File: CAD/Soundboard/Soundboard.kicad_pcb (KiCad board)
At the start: 2 copper layers, 105 x 85 mm, 53 parts, among them J1 USB4085-GF-A_REVB, Q1 IRLML6401, Q2 IRLML6401, Q3 IRLML6401, Q4 IRLML6401, SW1 SW_SPST, SW10 SW_SPST, SW11 SW_SPST, SW12 SW_SPST, SW13 SW_SPST, SW14 SW_SPST, SW15 SW_SPST, SW16 SW_SPST, SW2 SW_SPST, SW3 SW_SPST, SW4 SW_SPST, SW5 SW_SPST, SW6 SW_SPST, SW7 SW_SPST, SW8 SW_SPST, SW9 SW_SPST, U1 TLC59283DBQ

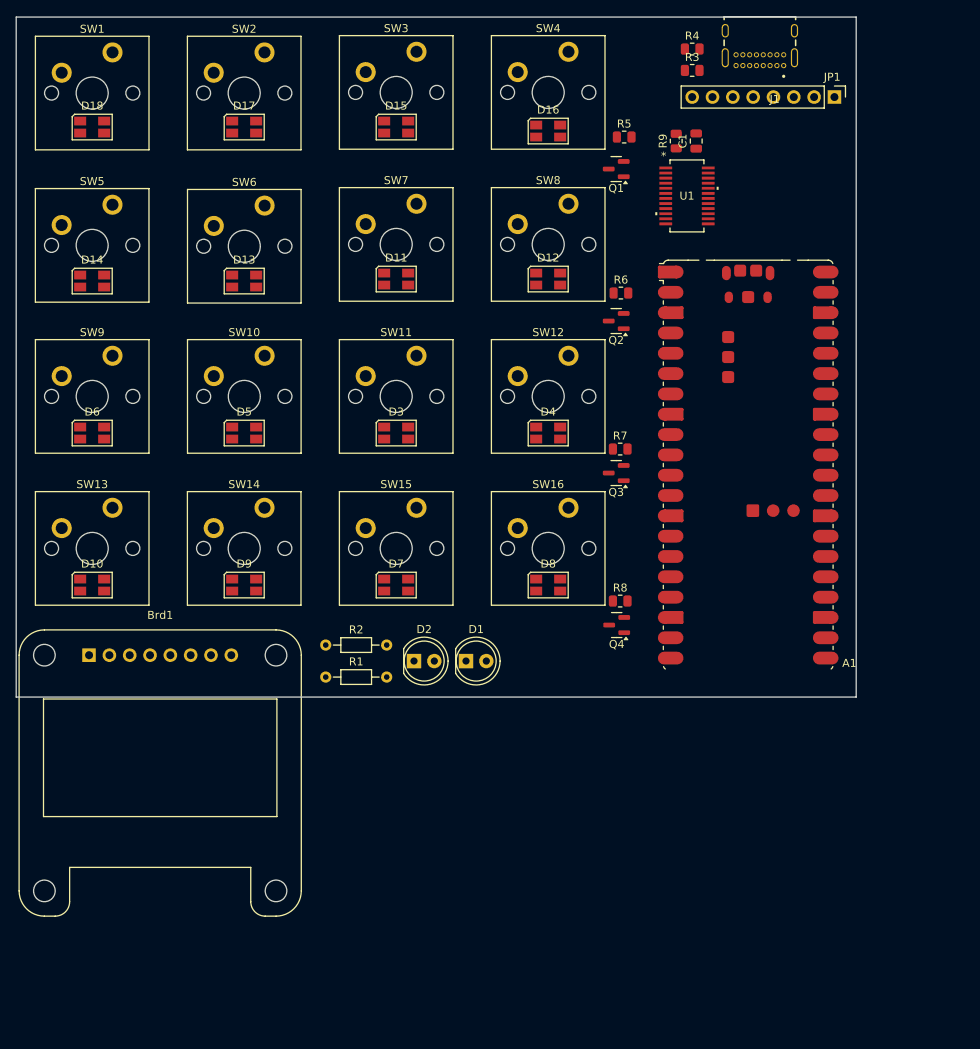
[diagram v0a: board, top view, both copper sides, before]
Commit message: do all the things
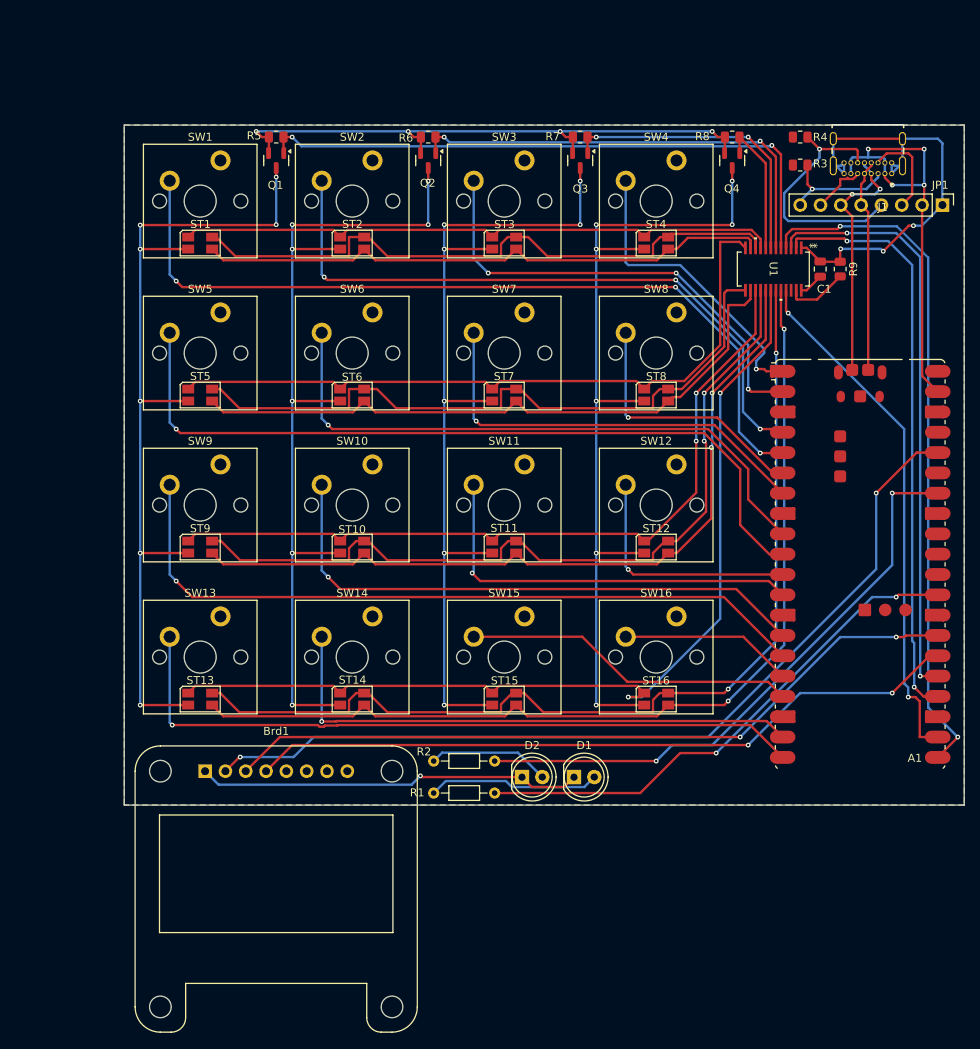
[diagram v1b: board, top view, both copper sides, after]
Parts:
- C1: value I dont know something big -> big
- J1: value USB4085-GF-A_REVB -> USB-C
- Q1, Q2: value IRLML6401 -> FET
- moved ST13 72.8 mm to (38.0, 100.2)
- moved ST16 71.9 mm to (95.0, 100.2)
- moved ST14 61.5 mm to (57.0, 100.2)
- moved ST15 61.3 mm to (76.0, 100.2)
- moved Q4 59.8 mm to (104.5, 32.9), turned to -90 degrees
- moved R8 59.7 mm to (104.5, 30.0)
- moved ST5 54.6 mm to (38.0, 62.2)
- moved ST4 53.7 mm to (95.0, 43.2)
- moved ST9 52.8 mm to (38.0, 81.2)
- moved ST12 51.7 mm to (95.0, 81.2)
- moved R5 43.5 mm to (47.5, 30.0)
- moved Q1 42.5 mm to (47.5, 32.9), turned to -90 degrees
- moved Q3 39.3 mm to (85.5, 32.9), turned to -90 degrees
- moved R7 39.3 mm to (85.5, 30.0)
- moved ST10 35.9 mm to (57.0, 81.2)
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- renumbered D15 to ST1, D13 to ST10, D5 to ST11, D9 to ST12, D18 to ST13, D14 to ST14, D6 to ST15, D10 to ST16, D11 to ST2, D3 to ST3, D7 to ST4, D16 to ST5, D12 to ST6, D4 to ST7, D8 to ST8, D17 to ST9
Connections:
- ST1 pad 1: Net-(D11-RK) -> Net-(ST1-RK)
- ST1 pad 2: Net-(D11-GK) -> Net-(ST1-GK)
- ST1 pad 3: Net-(D11-BK) -> Net-(ST1-BK)
- ST10 pad 1: Net-(D13-RK) -> Net-(ST10-RK)
- ST10 pad 2: Net-(D13-GK) -> Net-(ST10-GK)
- ST10 pad 3: Net-(D13-BK) -> Net-(ST10-BK)
- ST11 pad 1: Net-(D13-RK) -> Net-(ST10-RK)
- ST11 pad 2: Net-(D13-GK) -> Net-(ST10-GK)
- ST11 pad 3: Net-(D13-BK) -> Net-(ST10-BK)
- ST12 pad 1: Net-(D13-RK) -> Net-(ST10-RK)
- ST12 pad 2: Net-(D13-GK) -> Net-(ST10-GK)
- ST12 pad 3: Net-(D13-BK) -> Net-(ST10-BK)
- ST13 pad 1: Net-(D10-RK) -> Net-(ST13-RK)
- ST13 pad 2: Net-(D10-GK) -> Net-(ST13-GK)
- ST13 pad 3: Net-(D10-BK) -> Net-(ST13-BK)
- ST14 pad 1: Net-(D10-RK) -> Net-(ST13-RK)
- ST14 pad 2: Net-(D10-GK) -> Net-(ST13-GK)
- ST14 pad 3: Net-(D10-BK) -> Net-(ST13-BK)
- ST15 pad 1: Net-(D10-RK) -> Net-(ST13-RK)
- ST15 pad 2: Net-(D10-GK) -> Net-(ST13-GK)
- ST15 pad 3: Net-(D10-BK) -> Net-(ST13-BK)
- ST16 pad 1: Net-(D10-RK) -> Net-(ST13-RK)
- ST16 pad 2: Net-(D10-GK) -> Net-(ST13-GK)
- ST16 pad 3: Net-(D10-BK) -> Net-(ST13-BK)
- ST2 pad 1: Net-(D11-RK) -> Net-(ST1-RK)
- ST2 pad 2: Net-(D11-GK) -> Net-(ST1-GK)
- ST2 pad 3: Net-(D11-BK) -> Net-(ST1-BK)
- ST3 pad 1: Net-(D11-RK) -> Net-(ST1-RK)
- ST3 pad 2: Net-(D11-GK) -> Net-(ST1-GK)
- ST3 pad 3: Net-(D11-BK) -> Net-(ST1-BK)
- ST4 pad 1: Net-(D11-RK) -> Net-(ST1-RK)
- ST4 pad 2: Net-(D11-GK) -> Net-(ST1-GK)
- ST4 pad 3: Net-(D11-BK) -> Net-(ST1-BK)
- ST5 pad 1: Net-(D12-RK) -> Net-(ST5-RK)
- ST5 pad 2: Net-(D12-GK) -> Net-(ST5-GK)
- ST5 pad 3: Net-(D12-BK) -> Net-(ST5-BK)
- ST6 pad 1: Net-(D12-RK) -> Net-(ST5-RK)
- ST6 pad 2: Net-(D12-GK) -> Net-(ST5-GK)
- ST6 pad 3: Net-(D12-BK) -> Net-(ST5-BK)
- ST7 pad 1: Net-(D12-RK) -> Net-(ST5-RK)
- ST7 pad 2: Net-(D12-GK) -> Net-(ST5-GK)
- ST7 pad 3: Net-(D12-BK) -> Net-(ST5-BK)
- ST8 pad 1: Net-(D12-RK) -> Net-(ST5-RK)
- ST8 pad 2: Net-(D12-GK) -> Net-(ST5-GK)
- ST8 pad 3: Net-(D12-BK) -> Net-(ST5-BK)
- ST9 pad 1: Net-(D13-RK) -> Net-(ST10-RK)
- ST9 pad 2: Net-(D13-GK) -> Net-(ST10-GK)
- ST9 pad 3: Net-(D13-BK) -> Net-(ST10-BK)
- SW1 pad 1: /GPIO0 -> /GPIO3
- SW10 pad 1: /GPIO9 -> /GPIO10
- SW11 pad 1: /GPIO10 -> /GPIO9
- SW12 pad 1: /GPIO11 -> /GPIO8
- SW13 pad 1: /GPIO12 -> /GPIO15
- SW14 pad 1: /GPIO13 -> /GPIO14
- SW15 pad 1: /GPIO14 -> /GPIO13
- SW16 pad 1: /GPIO15 -> /GPIO12
- SW2 pad 1: /GPIO1 -> /GPIO2
- SW3 pad 1: /GPIO2 -> /GPIO1
- SW4 pad 1: /GPIO3 -> /GPIO0
- SW5 pad 1: /GPIO4 -> /GPIO7
- SW6 pad 1: /GPIO5 -> /GPIO6
- SW7 pad 1: /GPIO6 -> /GPIO5
- SW8 pad 1: /GPIO7 -> /GPIO4
- SW9 pad 1: /GPIO8 -> /GPIO11
- U1 pad 10: Net-(D10-GK) -> Net-(ST1-GK)
- U1 pad 11: Net-(D10-RK) -> Net-(ST1-BK)
- U1 pad 12: Net-(D13-BK) -> Net-(ST5-RK)
- U1 pad 13: Net-(D13-GK) -> Net-(ST5-GK)
- U1 pad 14: Net-(D13-RK) -> Net-(ST5-BK)
- U1 pad 15: Net-(D12-BK) -> Net-(ST10-RK)
- U1 pad 16: Net-(D12-GK) -> Net-(ST10-GK)
- U1 pad 17: Net-(D12-RK) -> Net-(ST10-BK)
- U1 pad 18: Net-(D11-BK) -> Net-(ST13-RK)
- U1 pad 19: Net-(D11-GK) -> Net-(ST13-GK)
- U1 pad 20: Net-(D11-RK) -> Net-(ST13-BK)
- U1 pad 9: Net-(D10-BK) -> Net-(ST1-RK)
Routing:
- net Net-(ST13-GK): track 0.00 -> 125.4 mm, vias 0 -> 2
- net Net-(ST13-BK): track 0.00 -> 122.6 mm, vias 0 -> 2
- net Net-(ST13-RK): track 0.00 -> 120.7 mm, vias 0 -> 2
- net /3V3: track 0.00 -> 111.1 mm, vias 0 -> 2
- net GND: track 0.00 -> 108.4 mm, vias 0 -> 4
- net Net-(Q4-D): track 0.00 -> 108.1 mm, vias 0 -> 7
- net Net-(Q3-D): track 0.00 -> 108.1 mm, vias 0 -> 7
- net Net-(Q2-D): track 0.00 -> 108.1 mm, vias 0 -> 7
- net Net-(Q1-D): track 0.00 -> 108.1 mm, vias 0 -> 7
- net /GPIO3: track 0.00 -> 103.6 mm, vias 0 -> 3
- net Net-(ST10-GK): track 0.00 -> 102.2 mm, vias 0 -> 2
- net Net-(ST10-BK): track 0.00 -> 99.0 mm, vias 0 -> 2
- net /GPIO7: track 0.00 -> 98.8 mm, vias 0 -> 1
- net Net-(ST10-RK): track 0.00 -> 96.6 mm, vias 0 -> 2
- net /SCREEN_SCL: track 0.00 -> 93.5 mm, vias 0 -> 2
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- added copper zone on B.Cu, net GND
- added copper zone on F.Cu, net GND
